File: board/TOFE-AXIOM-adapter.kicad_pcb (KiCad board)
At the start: 2 copper layers, 68.9 x 28.3 mm, 11 parts, among them CN1 C, U1 24AA01/24LC01B

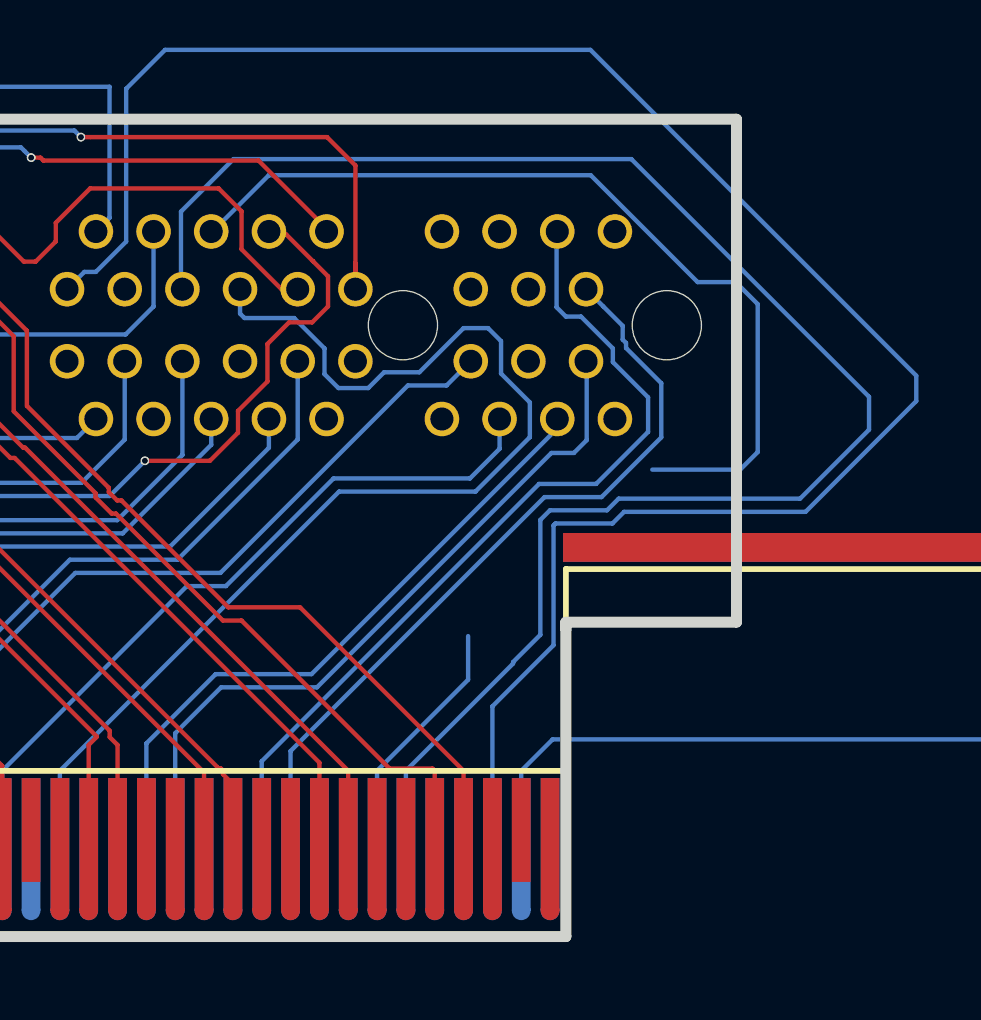
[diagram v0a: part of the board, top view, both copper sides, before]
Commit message: Small fix.
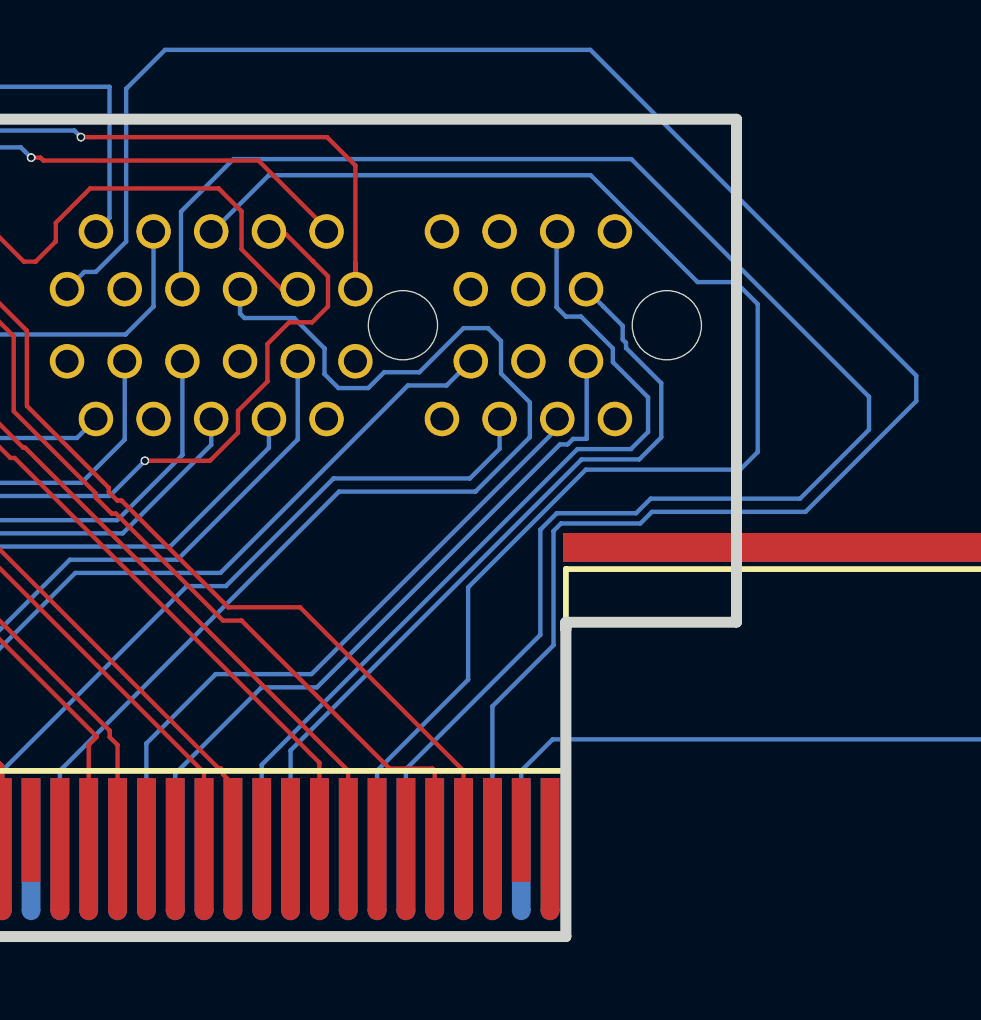
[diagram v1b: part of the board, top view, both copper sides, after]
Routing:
- net /S_IO2: track 39.3 -> 49.0 mm
- net /S_LVDS_4_N: track 25.0 -> 24.1 mm
